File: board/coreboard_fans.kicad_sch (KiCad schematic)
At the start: 8 parts

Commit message: Added most Footprints, Schematic review touch up
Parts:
- Conn2, Conn9: footprint (none) -> MRDT_Connectors:MOLEX_SL_04_Vertical
- R24, R25, R26, R27, R28, R29: footprint (none) -> Resistor_SMD:R_0603_1608Metric_Pad0.98x0.95mm_HandSolder
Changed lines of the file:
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@@
 			)
 		)
-		(property "Footprint" ""
+		(property "Footprint" "Resistor_SMD:R_0603_1608Metric_Pad0.98x0.95mm_HandSolder"
 			(at 151.9385 82.7303 90)
 			(effects
@@
 			)
 		)
-		(property "Footprint" ""
+		(property "Footprint" "MRDT_Connectors:MOLEX_SL_04_Vertical"
 			(at 194.1025 82.4763 0)
 			(effects
@@
 			)
 		)
-		(property "Footprint" ""
+		(property "Footprint" "Resistor_SMD:R_0603_1608Metric_Pad0.98x0.95mm_HandSolder"
 			(at 68.326 75.946 90)
 			(effects
@@
 			)
 		)
-		(property "Footprint" ""
+		(property "Footprint" "Resistor_SMD:R_0603_1608Metric_Pad0.98x0.95mm_HandSolder"
 			(at 61.976 81.534 90)
 			(effects
@@
 			)
 		)
-		(property "Footprint" ""
+		(property "Footprint" "Resistor_SMD:R_0603_1608Metric_Pad0.98x0.95mm_HandSolder"
 			(at 78.486 67.564 90)
 			(effects
@@
 			)
 		)
-		(property "Footprint" ""
+		(property "Footprint" "Resistor_SMD:R_0603_1608Metric_Pad0.98x0.95mm_HandSolder"
 			(at 158.2885 77.1423 90)
 			(effects
@@
 			)
 		)
-		(property "Footprint" ""
+		(property "Footprint" "Resistor_SMD:R_0603_1608Metric_Pad0.98x0.95mm_HandSolder"
 			(at 168.4485 68.7603 90)
 			(effects
@@
 			)
 		)
-		(property "Footprint" ""
+		(property "Footprint" "MRDT_Connectors:MOLEX_SL_04_Vertical"
 			(at 104.14 81.28 0)
 			(effects

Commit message: routed core board
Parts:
- Conn2, Conn9: footprint MRDT_Connectors:MOLEX_SL_04_Vertical -> MRDT_Connectors:MOLEX_SL_04_Horizontal
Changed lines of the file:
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@@
 			)
 		)
-		(property "Footprint" "MRDT_Connectors:MOLEX_SL_04_Vertical"
+		(property "Footprint" "MRDT_Connectors:MOLEX_SL_04_Horizontal"
 			(at 194.1025 82.4763 0)
 			(effects
@@
 			)
 		)
-		(property "Footprint" "MRDT_Connectors:MOLEX_SL_04_Vertical"
+		(property "Footprint" "MRDT_Connectors:MOLEX_SL_04_Horizontal"
 			(at 104.14 81.28 0)
 			(effects

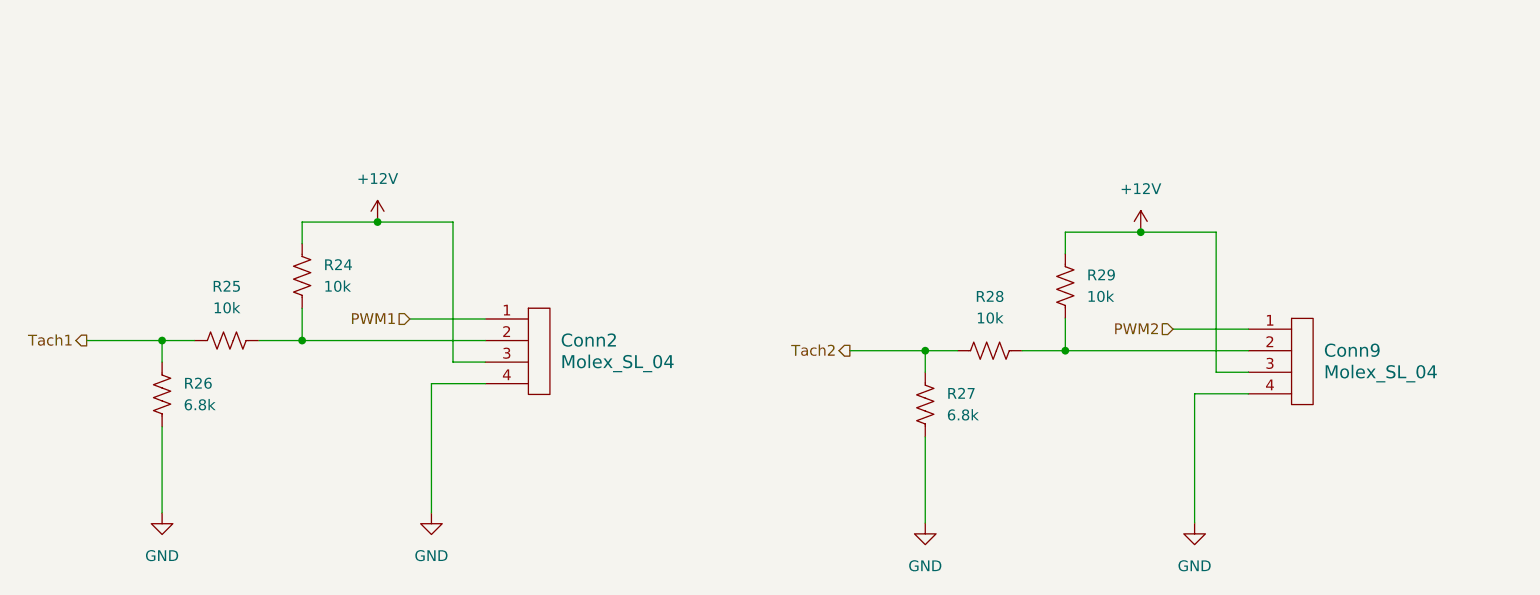
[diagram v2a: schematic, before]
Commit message: Preliminary changes for rev2
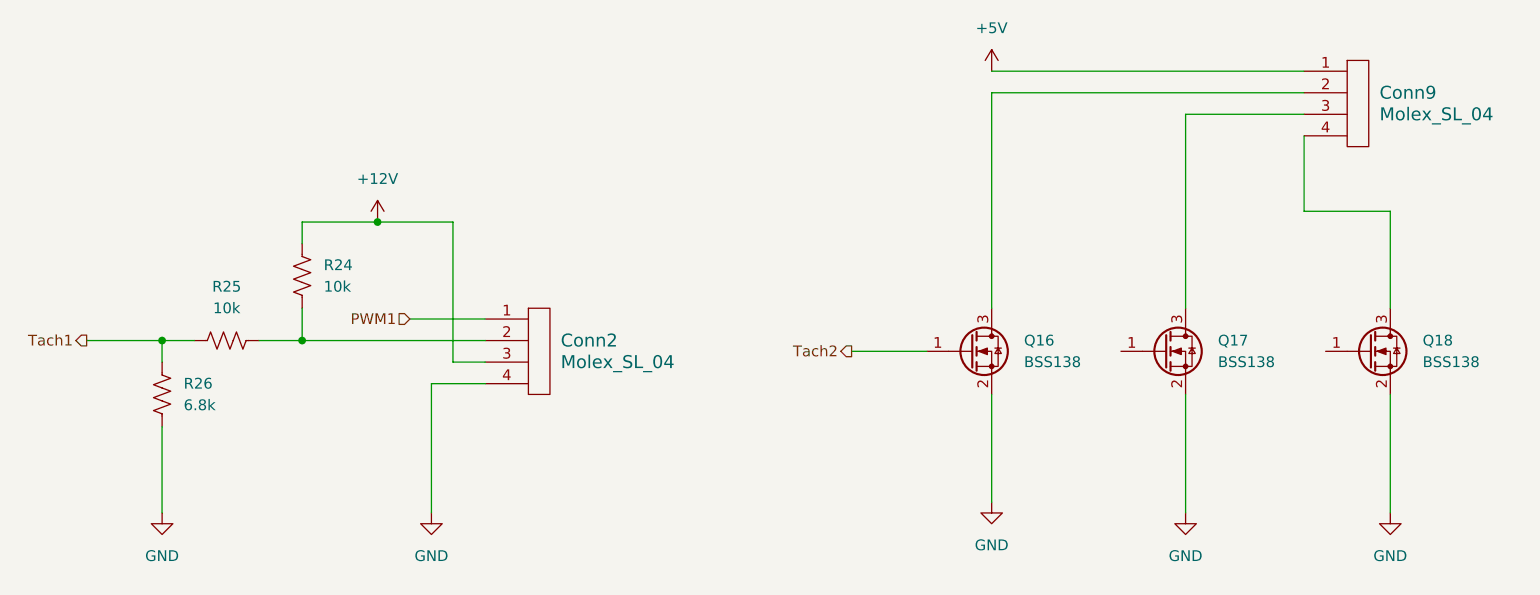
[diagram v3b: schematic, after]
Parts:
- removed R27: 6.8k, Resistor_SMD:R_0603_1608Metric_Pad0.98x0.95mm_HandSolder, symbol Device:R_US
- removed R28, R29: 10k, Resistor_SMD:R_0603_1608Metric_Pad0.98x0.95mm_HandSolder, symbol Device:R_US
- added Q16, Q17, Q18: BSS138, Package_TO_SOT_SMD:SOT-23, symbol Transistor_FET:BSS138
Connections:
- net +12V: no longer Conn9.3
- net GND: now also Q16.2 (S), Q17.2 (S), Q18.2 (S); no longer Conn9.4
- net Tach2: now also Q16.1 (G)
- net at Conn9.2: now also Q16.3 (D)
- net PWM2 renamed +5V
- new net: Conn9.3, Q17.3 (D)
- new net: Conn9.4, Q18.3 (D)
